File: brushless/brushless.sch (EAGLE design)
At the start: 71 parts, among them Q1 BUK7Y12-40E, Q2 BUK7Y12-40E, Q3 BUK7Y12-40E, Q4 BUK7Y12-40E, Q5 BUK7Y12-40E, Q6 BUK7Y12-40E, X2 MOTOR

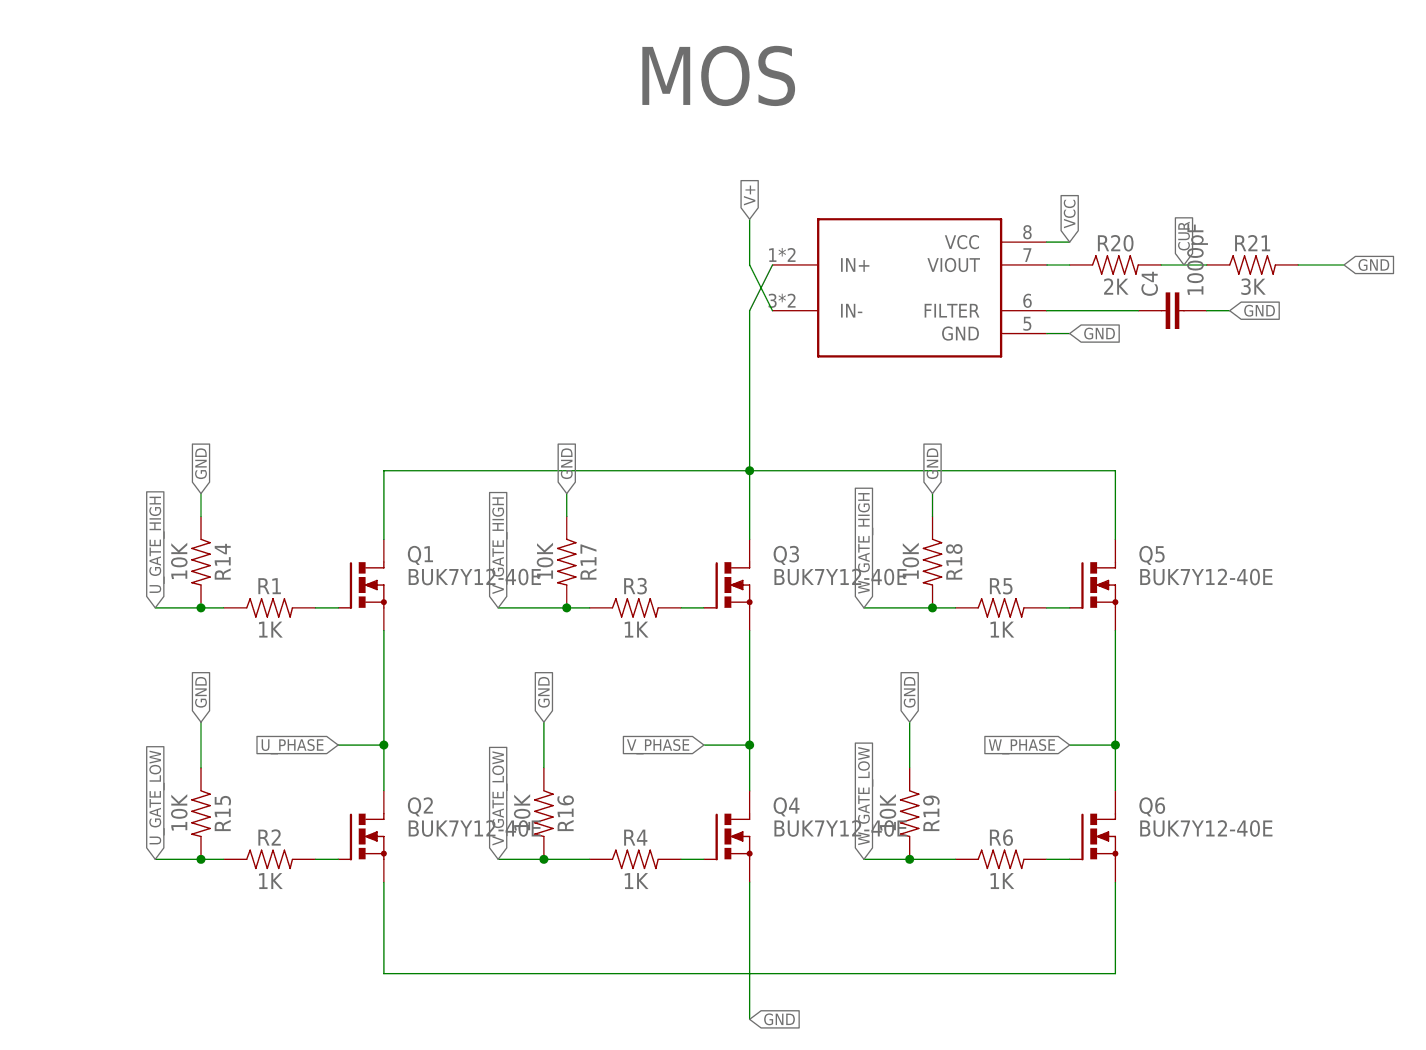
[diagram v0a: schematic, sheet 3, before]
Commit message: Updating designs
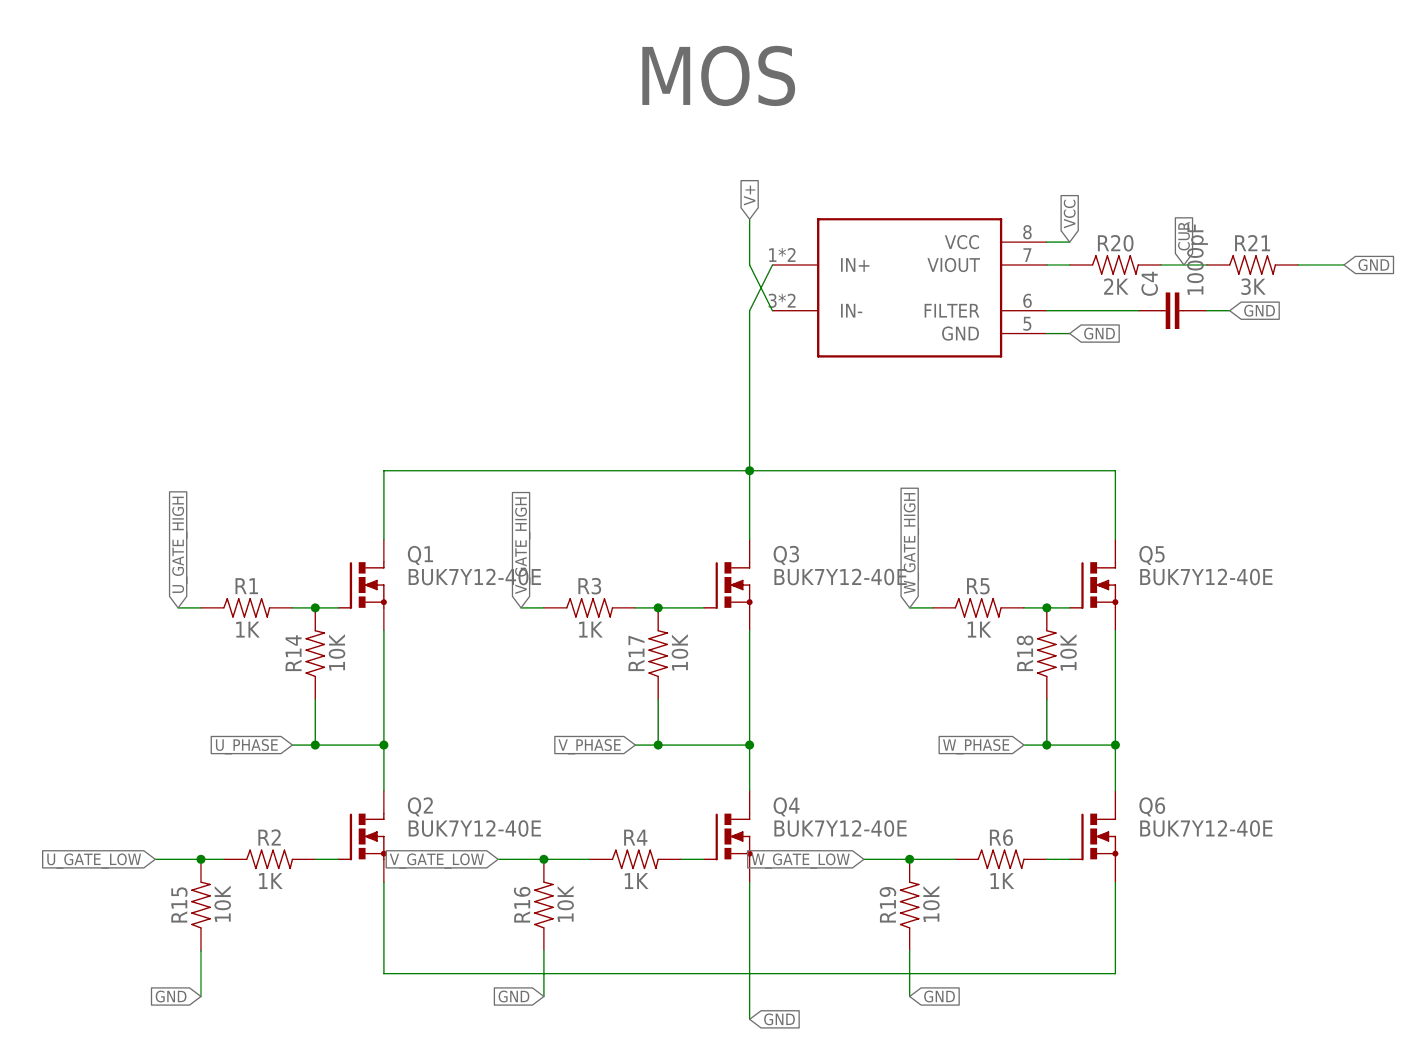
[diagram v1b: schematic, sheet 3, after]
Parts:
- removed R13, R22, R26: 10K, SparkFun-Resistors:RESISTOR0805
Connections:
- net GND: no longer R13.1, R14.1, R17.1, R18.1, R22.1, R26.1
- net HALLU: no longer R26.2
- net HALLV: no longer R22.2
- net HALLW: no longer R13.2
- net N$1: now also R14.2
- net N$2: now also R17.2
- net N$7: now also R18.2
- net U_GATE_HIGH: no longer R14.2
- net U_PHASE: now also R14.1
- net V_GATE_HIGH: no longer R17.2
- net V_PHASE: now also R17.1
- net W_GATE_HIGH: no longer R18.2
- net W_PHASE: now also R18.1
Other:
- moved on the sheet: R1, R14, R15, R16, R17, R18, R19, R3, R5
